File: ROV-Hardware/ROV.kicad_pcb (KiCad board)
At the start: 2 copper layers, 130 x 90 mm, 30 parts, among them J1 T-block, J2 Screw_Terminal_01x04, J3 Screw_Terminal_01x04, J4 T-block, U1 LM2596, U3 ESP32-S3-DEVKITC-1-N8R2, U4 MPU6050, U5 ZK-BM1, U6 ZK-BM1, U7 ZK-BM1, U8 A4988, U9 GY-MS5837

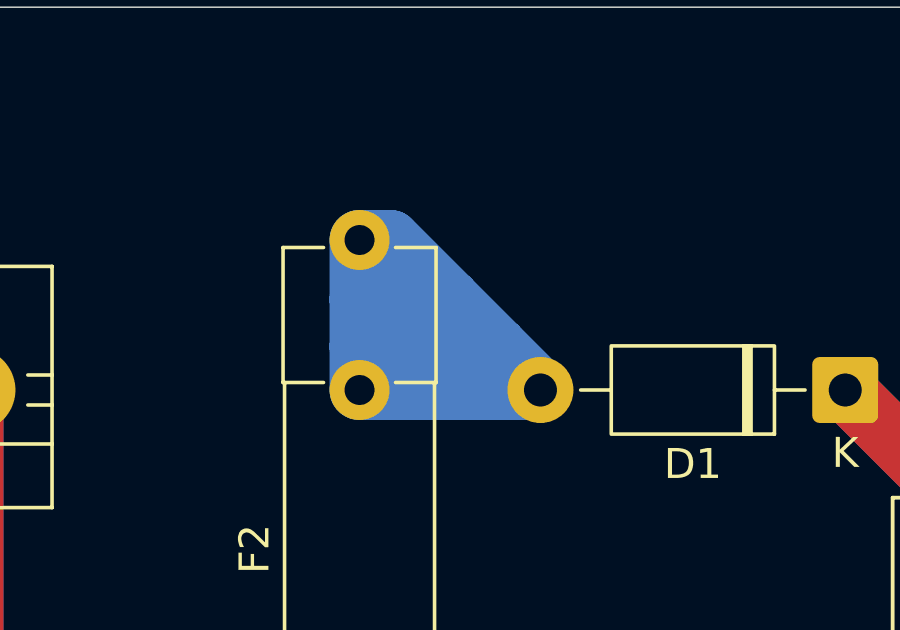
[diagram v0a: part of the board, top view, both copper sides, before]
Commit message: refresh
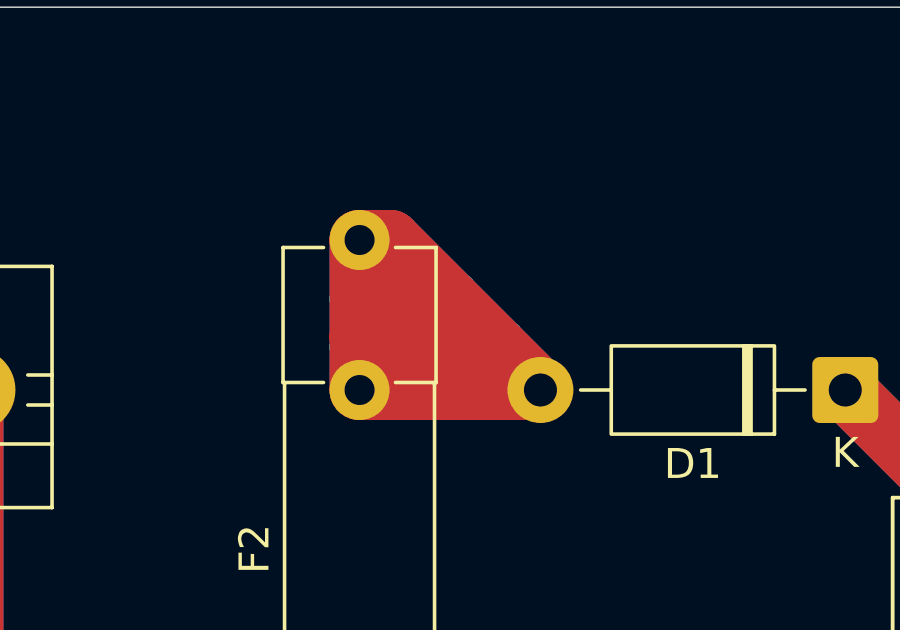
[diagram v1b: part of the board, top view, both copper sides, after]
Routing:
- net Net-(D1-A): track 26.7 -> 57.2 mm
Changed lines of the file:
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@@
 		(tenting front back)
 		(pcbplotparams
-			(layerselection 0x00000000_00000000_55555555_55555551)
+			(layerselection 0x00000000_00000000_55555555_55555555)
 			(plot_on_all_layers_selection 0x00000000_00000000_00000000_00000000)
 			(disableapertmacros no)
@@
 			(dxfimperialunits yes)
 			(dxfusepcbnewfont yes)
-			(psnegative no)
+			(psnegative yes)
 			(psa4output no)
 			(plot_black_and_white yes)
@@
 			(subtractmaskfromsilk no)
 			(outputformat 4)
-			(mirror no)
+			(mirror yes)
 			(drillshape 2)
 			(scaleselection 1)
@@
 	)
 	(segment
+		(start 162.33 67.315)
+		(end 160.575 65.56)
+		(width 2)
+		(layer "F.Cu")
+		(net 16)
+	)
+	(segment
+		(start 160.575 65.56)
+		(end 157.33 62.315)
+		(width 2)
+		(layer "F.Cu")
+		(net 16)
+	)
+	(segment
+		(start 163.36 67.315)
+		(end 162.33 67.315)
+		(width 2)
+		(layer "F.Cu")
+		(net 16)
+	)
+	(segment
+		(start 157.33 62.315)
+		(end 158.36 62.315)
+		(width 2)
+		(layer "F.Cu")
+		(net 16)
+	)
+	(segment
+		(start 157.33 65.56)
+		(end 157.33 62.315)
+		(width 2)
+		(layer "F.Cu")
+		(net 16)
+	)
+	(segment
+		(start 157.33 65.56)
+		(end 160.575 65.56)
+		(width 2)
+		(layer "F.Cu")
+		(net 16)
+	)
+	(segment
+		(start 157.33 67.315)
+		(end 157.33 65.56)
+		(width 2)
+		(layer "F.Cu")
+		(net 16)
+	)
+	(segment
+		(start 157.33 67.315)
+		(end 163.36 67.315)
+		(width 2)
+		(layer "F.Cu")
+		(net 16)
+	)
+	(segment
+		(start 158.36 62.315)
+		(end 163.36 67.315)
+		(width 2)
+		(layer "F.Cu")
+		(net 16)
+	)
+	(segment
